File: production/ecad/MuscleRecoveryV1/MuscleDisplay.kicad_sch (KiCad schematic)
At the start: 2 parts, among them J6 Conn_01x11_Pin

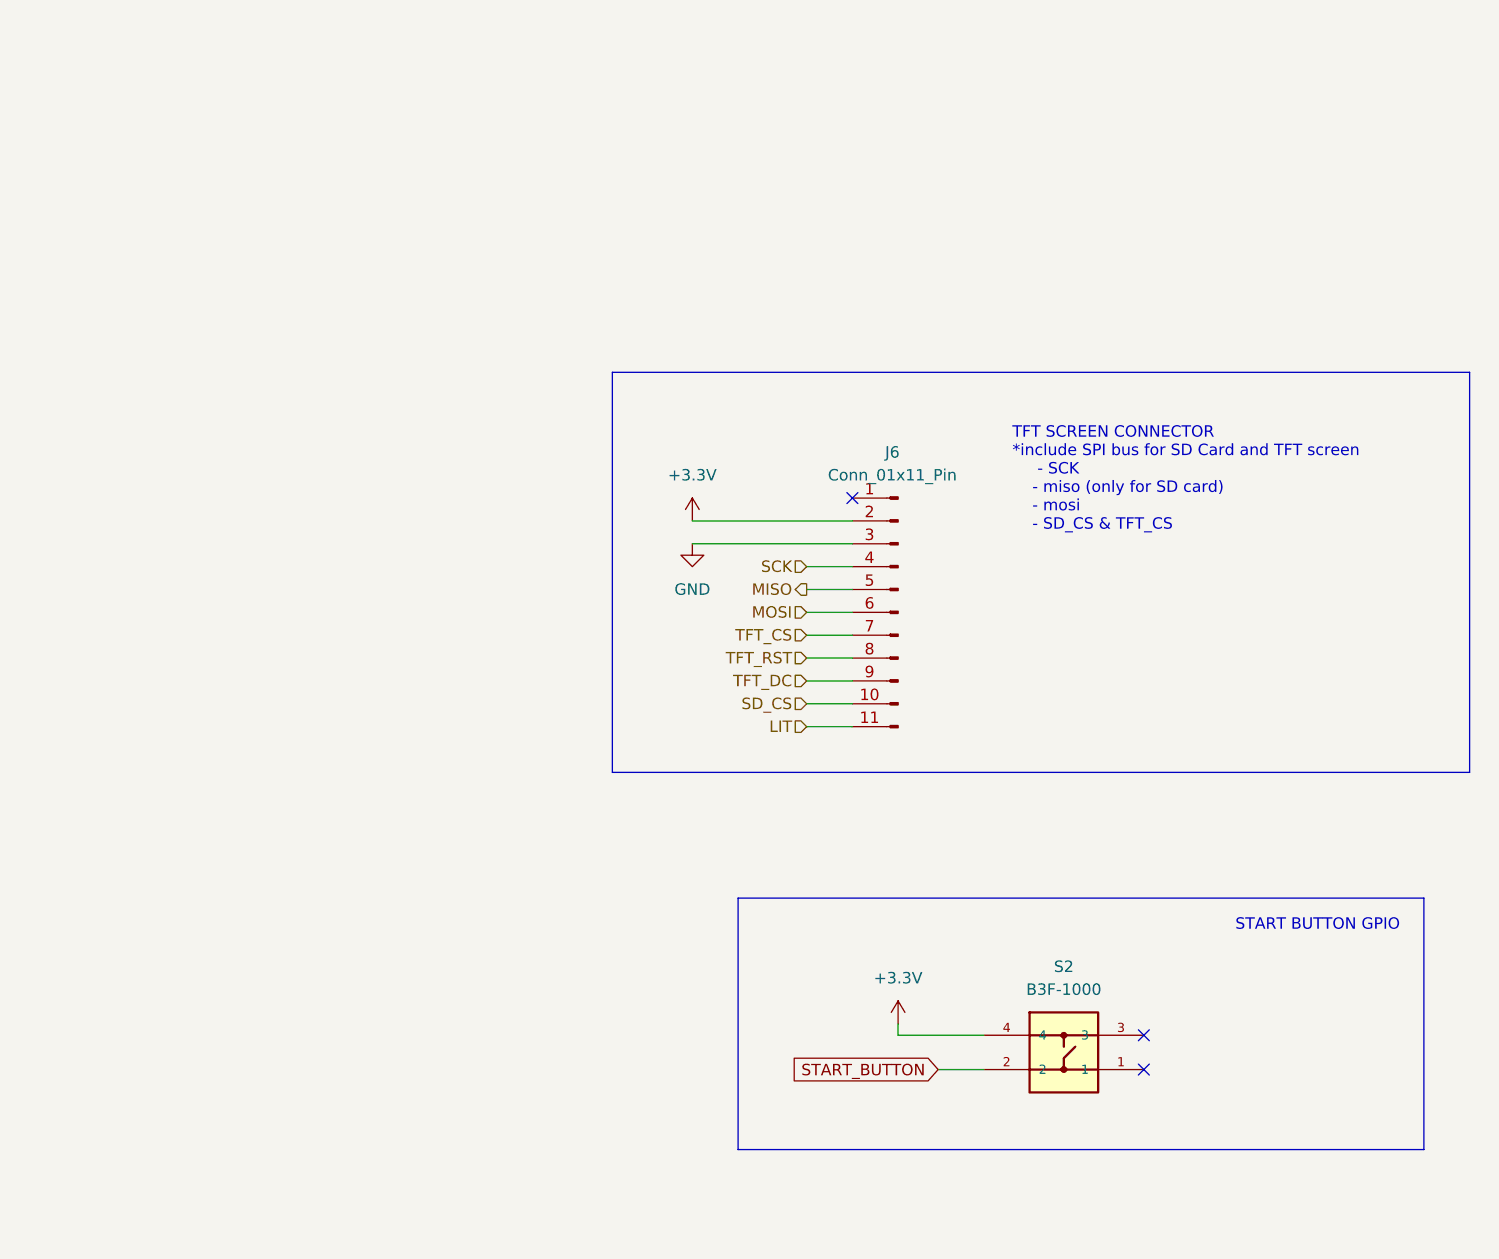
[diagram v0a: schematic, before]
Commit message: Maggie fixing her mistakes lol
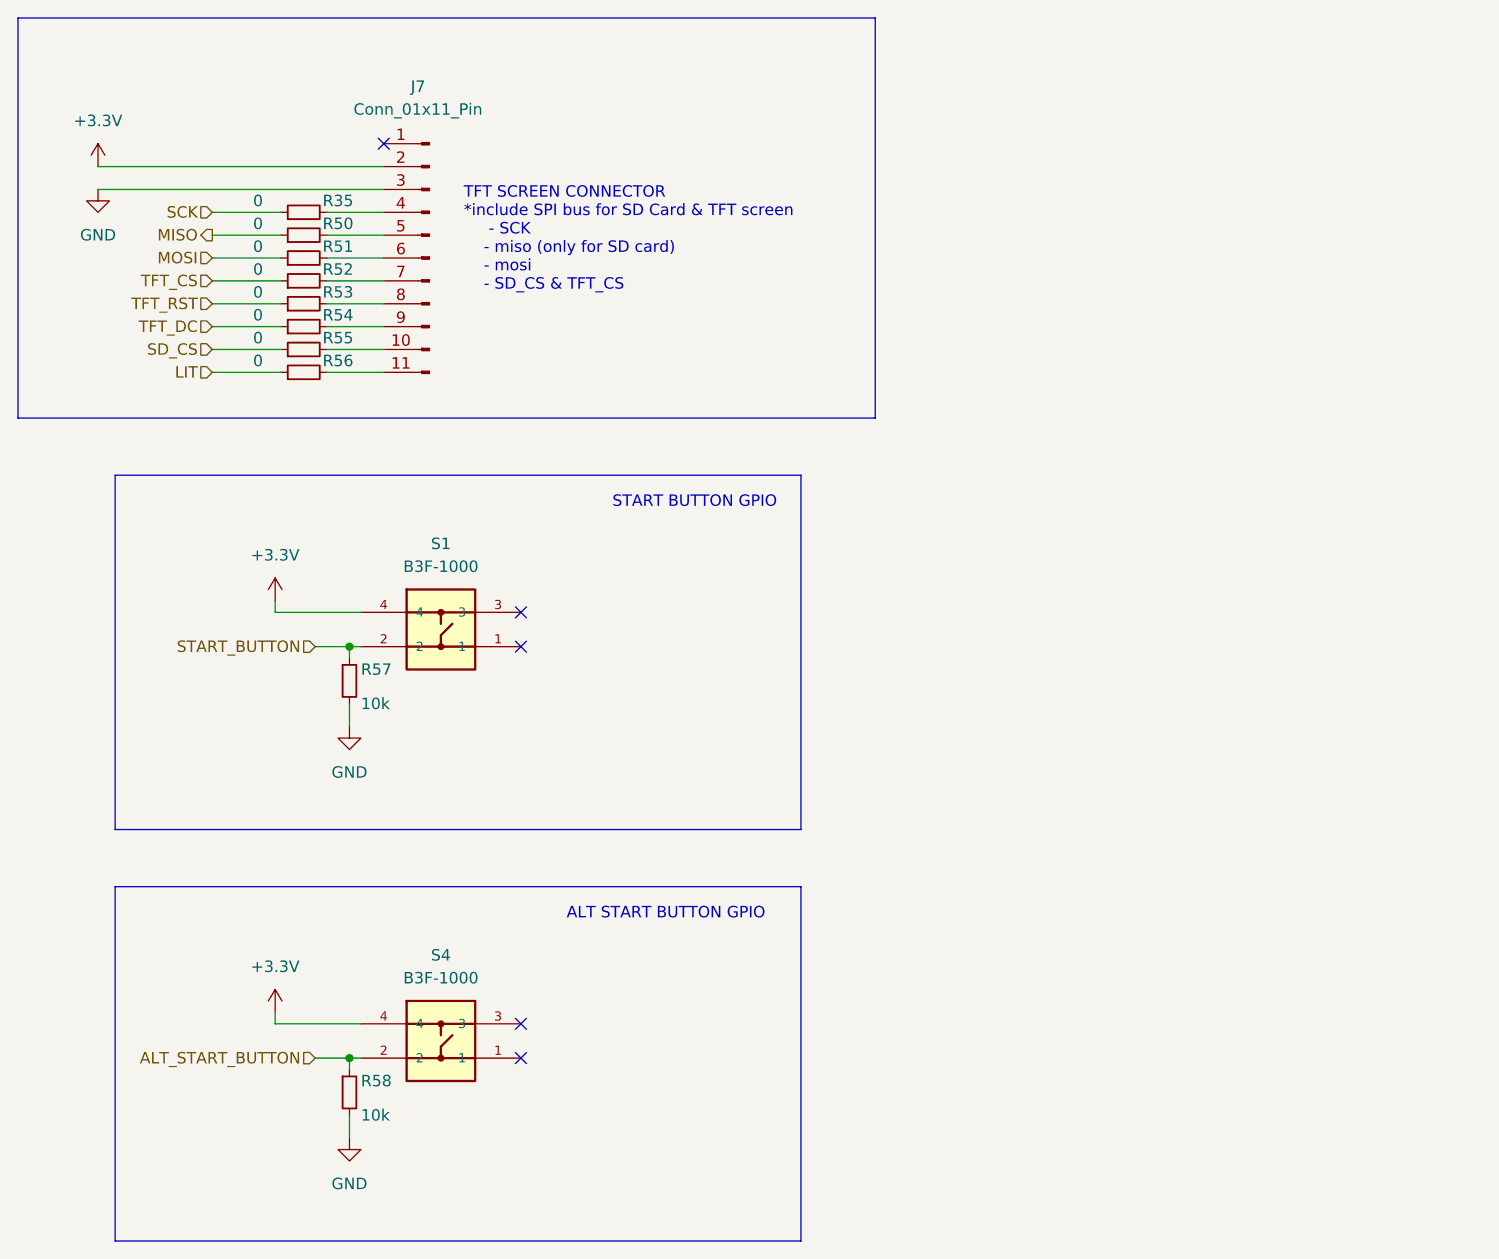
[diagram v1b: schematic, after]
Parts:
- removed J6: Conn_01x11_Pin, symbol Connector:Conn_01x11_Pin
- added J7: Conn_01x11_Pin, symbol Connector:Conn_01x11_Pin
- added R35, R50, R51, R52, R53, R54, R55, R56: 0, symbol Device:R_Small
- added R57, R58: 10k, symbol Device:R_Small
- added S4: B3F-1000, B3F-1000:SW_B3F-1000, symbol B3F-1000:B3F-1000
- renumbered S2 to S1
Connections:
- net +3.3V: now also J7.2 (Pin_2), S4.4
- net GND: now also J7.3 (Pin_3), R57.2, R58.2
- net LIT: now also R56.1
- net MISO: now also R50.1
- net MOSI: now also R51.1
- net SCK: now also R35.1
- net SD_CS: now also R55.1
- net START_BUTTON: now also R57.1
- net TFT_CS: now also R52.1
- net TFT_DC: now also R54.1
- net TFT_RST: now also R53.1
- new net: J7.4 (Pin_4), R35.2
- new net: J7.11 (Pin_11), R56.2
- new net: J7.8 (Pin_8), R53.2
- new net: J7.7 (Pin_7), R52.2
- new net: J7.9 (Pin_9), R54.2
- new net: J7.5 (Pin_5), R50.2
- new net: J7.10 (Pin_10), R55.2
- new net: J7.6 (Pin_6), R51.2
- new net ALT_START_BUTTON: R58.1, S4.2
- no-connect marks 3 -> 5
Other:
- note added: "ALT START BUTTON GPIO"
- note added: "TFT SCREEN CONNECTOR *include SPI bus for SD Card & TFT screen - SCK - miso (only for SD card) - mosi - SD_CS & TFT_CS"
- note removed: "TFT SCREEN CONNECTOR *include SPI bus for SD Card and TFT screen - SCK - miso (only for SD card) - mosi - SD_CS & TFT_CS"
- moved on the sheet: S1
